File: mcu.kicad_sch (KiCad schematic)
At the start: 1 part, among them U1 STM32F446VETx

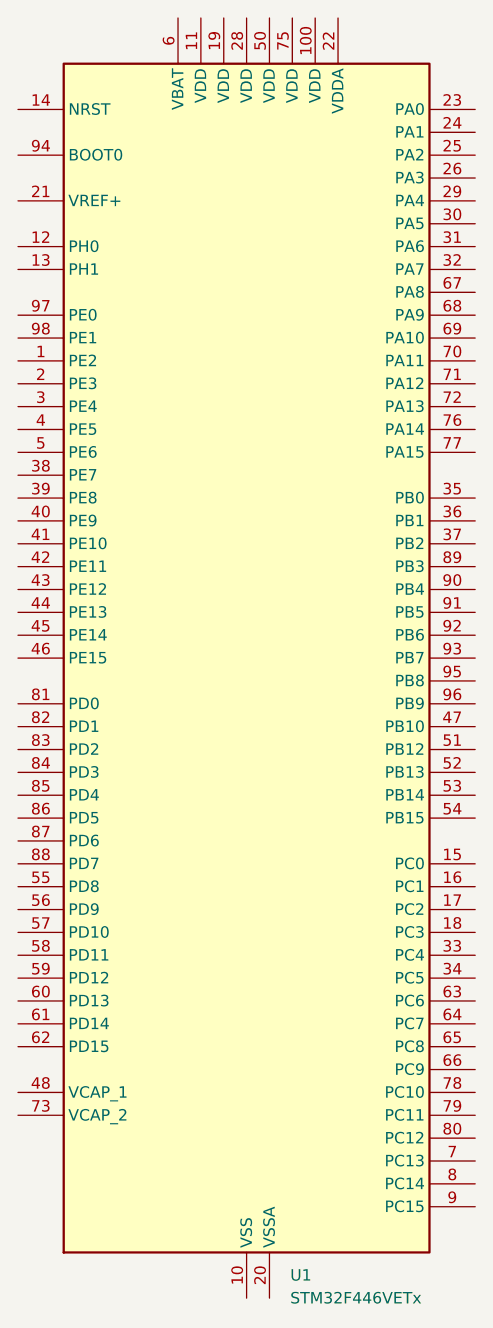
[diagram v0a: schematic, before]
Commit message: Power rail stuff
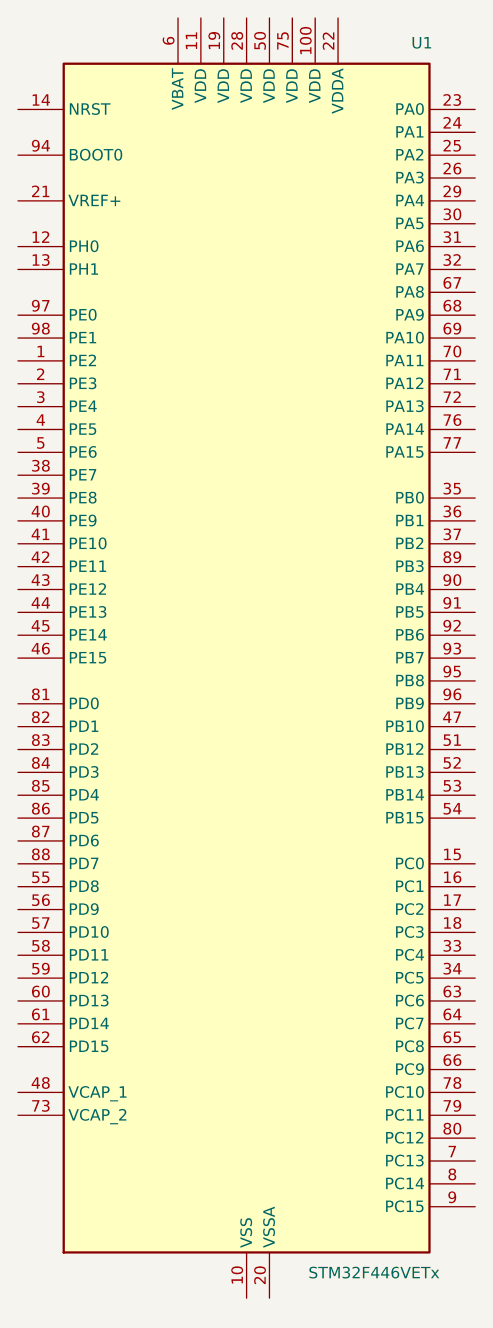
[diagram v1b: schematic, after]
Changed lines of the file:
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@@
 		(in_pos_files yes)
 		(dnp no)
-		(fields_autoplaced yes)
 		(property "Reference" "U1"
-			(at 135.6548 172.72 0)
+			(at 149.098 35.814 0)
 			(show_name no)
 			(do_not_autoplace no)
@@
 		)
 		(property "Value" "STM32F446VETx"
-			(at 135.6548 175.26 0)
+			(at 137.668 172.466 0)
 			(show_name no)
 			(do_not_autoplace no)
@@
 		(instances
 			(project "modretrocon"
-				(path "/4f4dfd23-e96d-40a8-91c2-e53fb8a1f2eb"
-					(reference "U1")
-					(unit 1)
-				)
-			)
-			(project "modretrocon"
 				(path "/cf6749e4-132f-4e26-b0d6-92782ee54bed/4d59c3d8-a5c2-4135-9570-fdfaf506da3f"
